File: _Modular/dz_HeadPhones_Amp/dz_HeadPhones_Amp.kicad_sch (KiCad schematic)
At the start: 83 parts, among them J1 In, J2 Through, J3 Power, J4 ModPower, J5 Phones, J6 Meter R, J7 Meter L, Q1 КТ503, Q2 КТ502, Q3 КТ503, Q4 КТ502, U1 TL072, U2 TL084

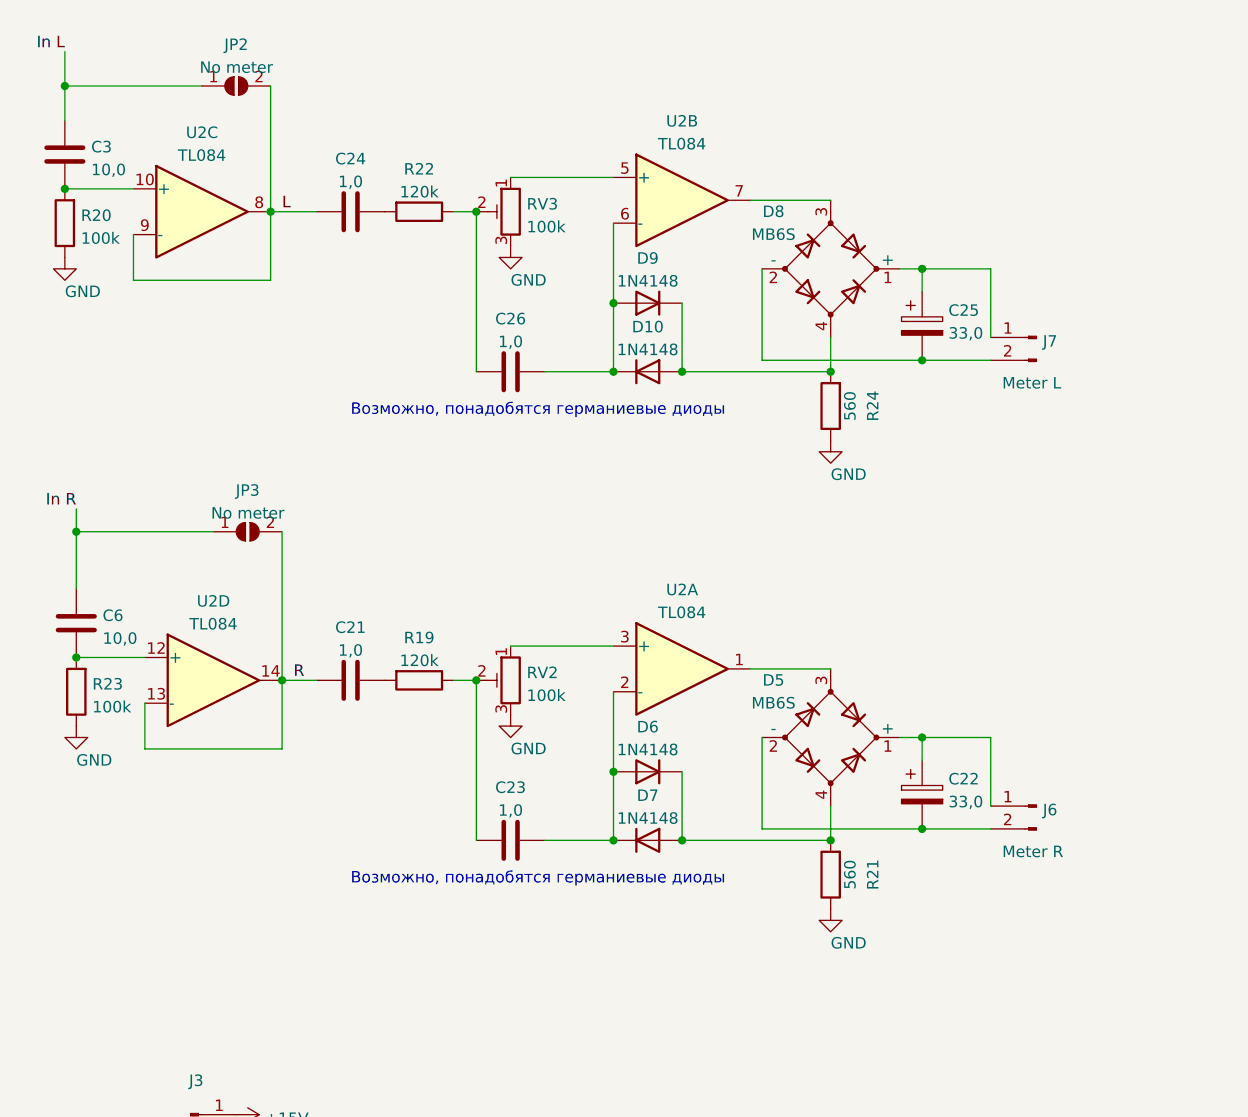
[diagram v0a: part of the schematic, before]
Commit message: meter
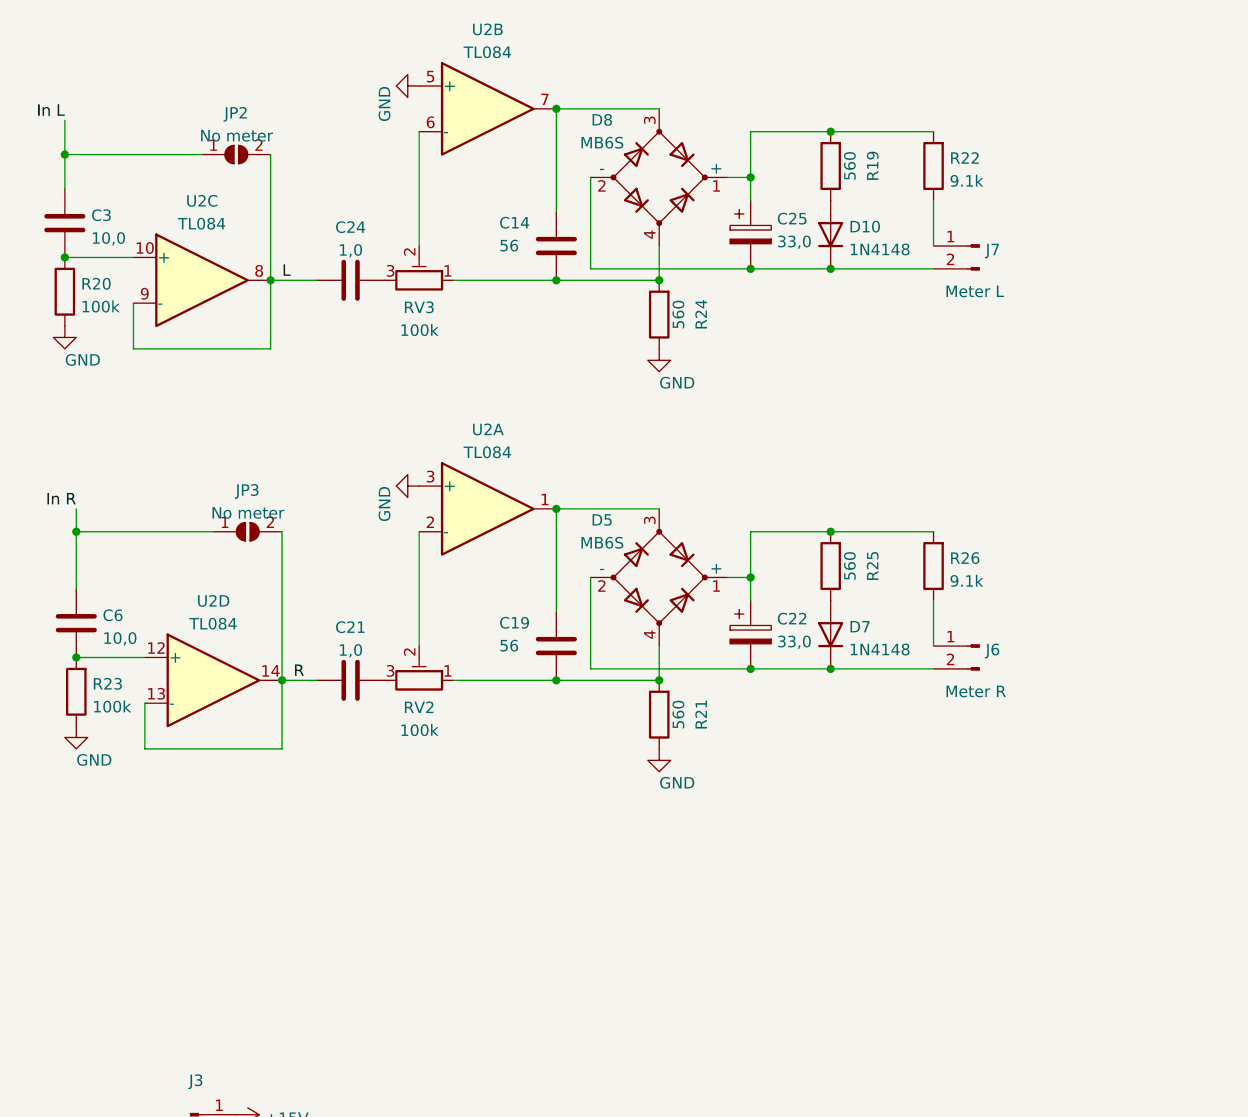
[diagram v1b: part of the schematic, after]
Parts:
- removed C23, C26: 1,0, Capacitor_SMD:C_0805_2012Metric_Pad1.18x1.45mm_HandSolder, symbol Device:C
- removed D6, D9: 1N4148, Diode_THT:D_DO-35_SOD27_P2.54mm_Vertical_KathodeUp, symbol Diode:1N4148
- added C14, C19: 56, Capacitor_THT:C_Disc_D5.0mm_W2.5mm_P2.50mm, symbol Device:C
- added R25: 560, Resistor_THT:R_Axial_DIN0207_L6.3mm_D2.5mm_P2.54mm_Vertical, symbol Device:R
- added R26: 9.1k, Resistor_THT:R_Axial_DIN0207_L6.3mm_D2.5mm_P2.54mm_Vertical, symbol Device:R
- R19: value 120k -> 560
- R22: value 120k -> 9.1k
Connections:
- net GND: now also U2.3 (+), U2.5 (+); no longer RV2.3, RV3.3
- net at C22.1, D5.1 (+): now also R25.2, R26.2; no longer J6.1 (Pin_1)
- net at C22.2, D5.2 (-), J6.2 (Pin_2): now also D7.1 (K)
- net at D5.3, U2.1: now also C19.1
- net at D5.4, R21.2: now also RV2.1, C19.2; no longer D7.2 (A)
- net at U2.2 (-): now also RV2.2; no longer D7.1 (K)
- net at RV3.1: now also D8.4, R24.2, C14.2; no longer U2.5 (+)
- net at RV3.2: now also U2.6 (-); no longer R22.1
- net at R19.1: now also D10.2 (A); no longer RV2.2
- net at C25.1, D8.1 (+): now also R19.2, R22.2; no longer J7.1 (Pin_1)
- net at C25.2, D8.2 (-), J7.2 (Pin_2): now also D10.1 (K)
- net at D8.3, U2.7: now also C14.1
- net at C24.2: now also RV3.3; no longer R22.2
- net at C21.2: now also RV2.3; no longer R19.2
- new net: D7.2 (A), R25.1
- new net: J7.1 (Pin_1), R22.1
- new net: J6.1 (Pin_1), R26.1
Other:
- note removed: "Возможно, понадобятся германиевые диоды"
- moved on the sheet: C22, C24, C25, C3, D10, D5, D7, D8, J6, J7, JP2, R20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
